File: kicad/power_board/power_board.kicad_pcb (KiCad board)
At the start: 2 copper layers, 98.4 x 77 mm, 54 parts, among them J1 24V, J10 Grid, J11 24V Solar, J2 24V, J3 GND, J4 GND, J5 GND, J6 GND, J7 MCU, J8 GND, J9 Solar Panel, Q1 FDD8453LZ, Q2 FDD8453LZ, Q3 FDD8453LZ, Q4 FDD8453LZ, Q5 FDS5670, U5 LT3757A, U6 LT1161

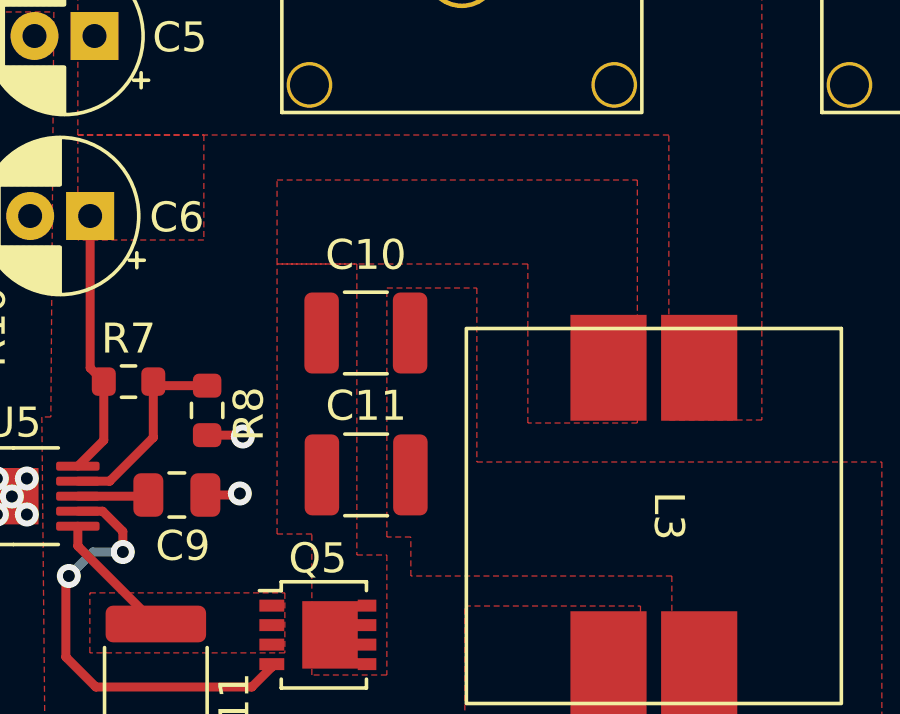
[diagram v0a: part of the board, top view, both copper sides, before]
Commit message: WIP
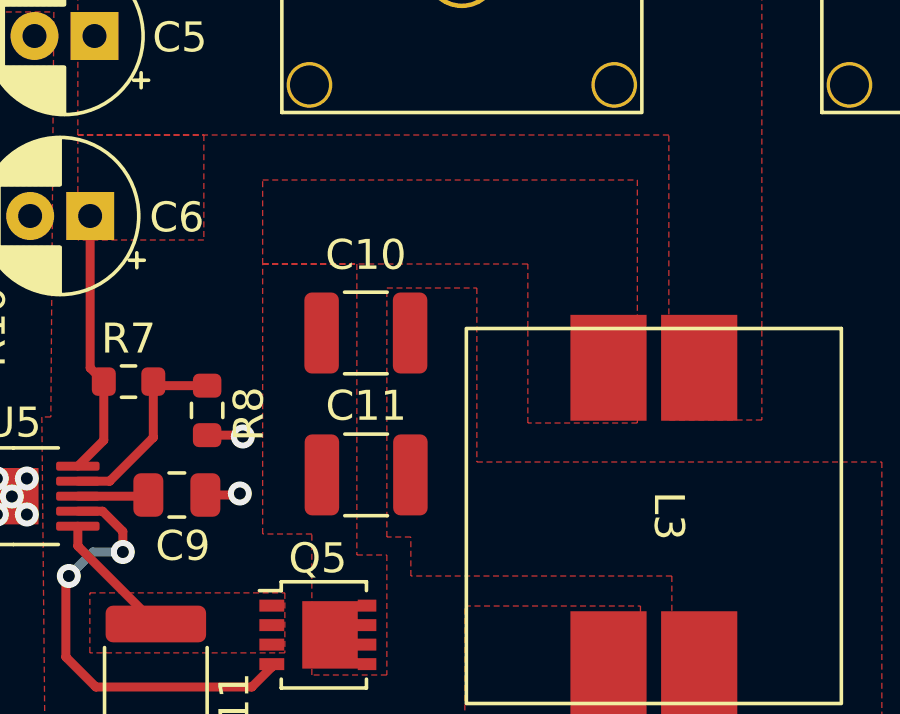
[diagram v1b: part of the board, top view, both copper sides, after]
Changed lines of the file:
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@@
         (xy 101.5 84.75)
         (xy 101.5 80.05)
-        (xy 100.34 80.05)
-        (xy 100.34 71.05)
+        (xy 99.86 80.05)
+        (xy 99.86 71.05)
         (xy 103 71.05)
       )
@@
         (xy 108.7 76.35)
         (xy 108.7 71.05)
-        (xy 100.34 71.05)
-        (xy 100.34 68.25)
+        (xy 99.86 71.05)
+        (xy 99.86 68.25)
         (xy 112.35 68.25)
       )
